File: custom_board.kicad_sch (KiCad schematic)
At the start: 20 parts, among them IC1 TMPM46BF10FG

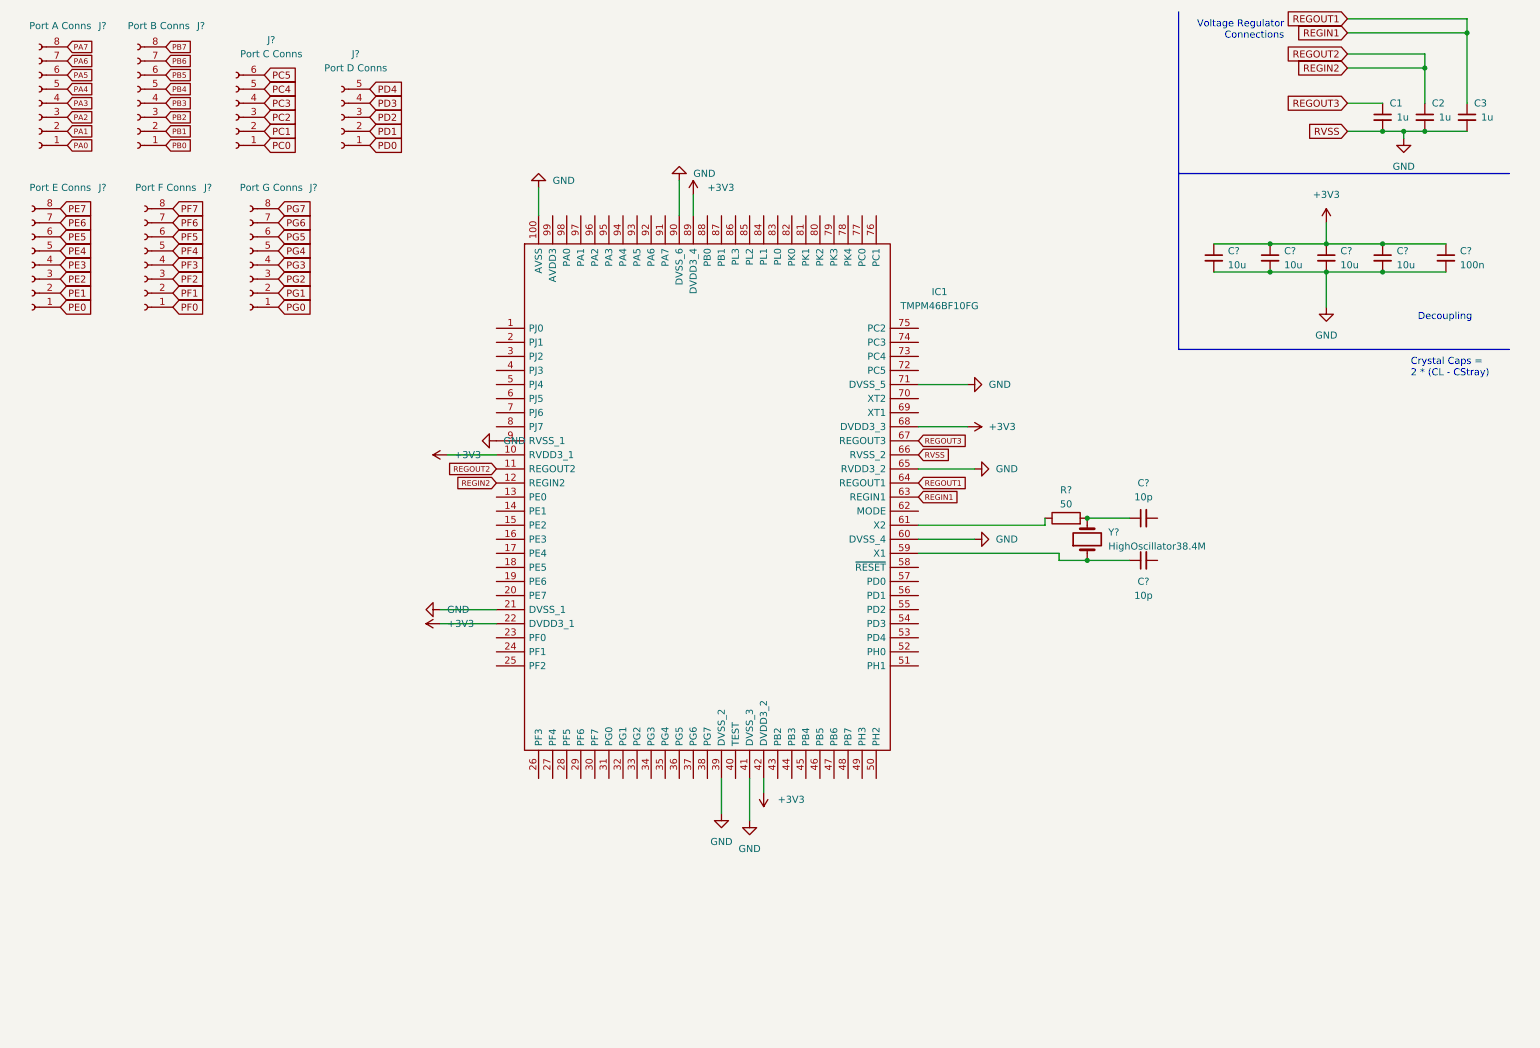
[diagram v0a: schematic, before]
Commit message: Update custom_board.kicad_sch
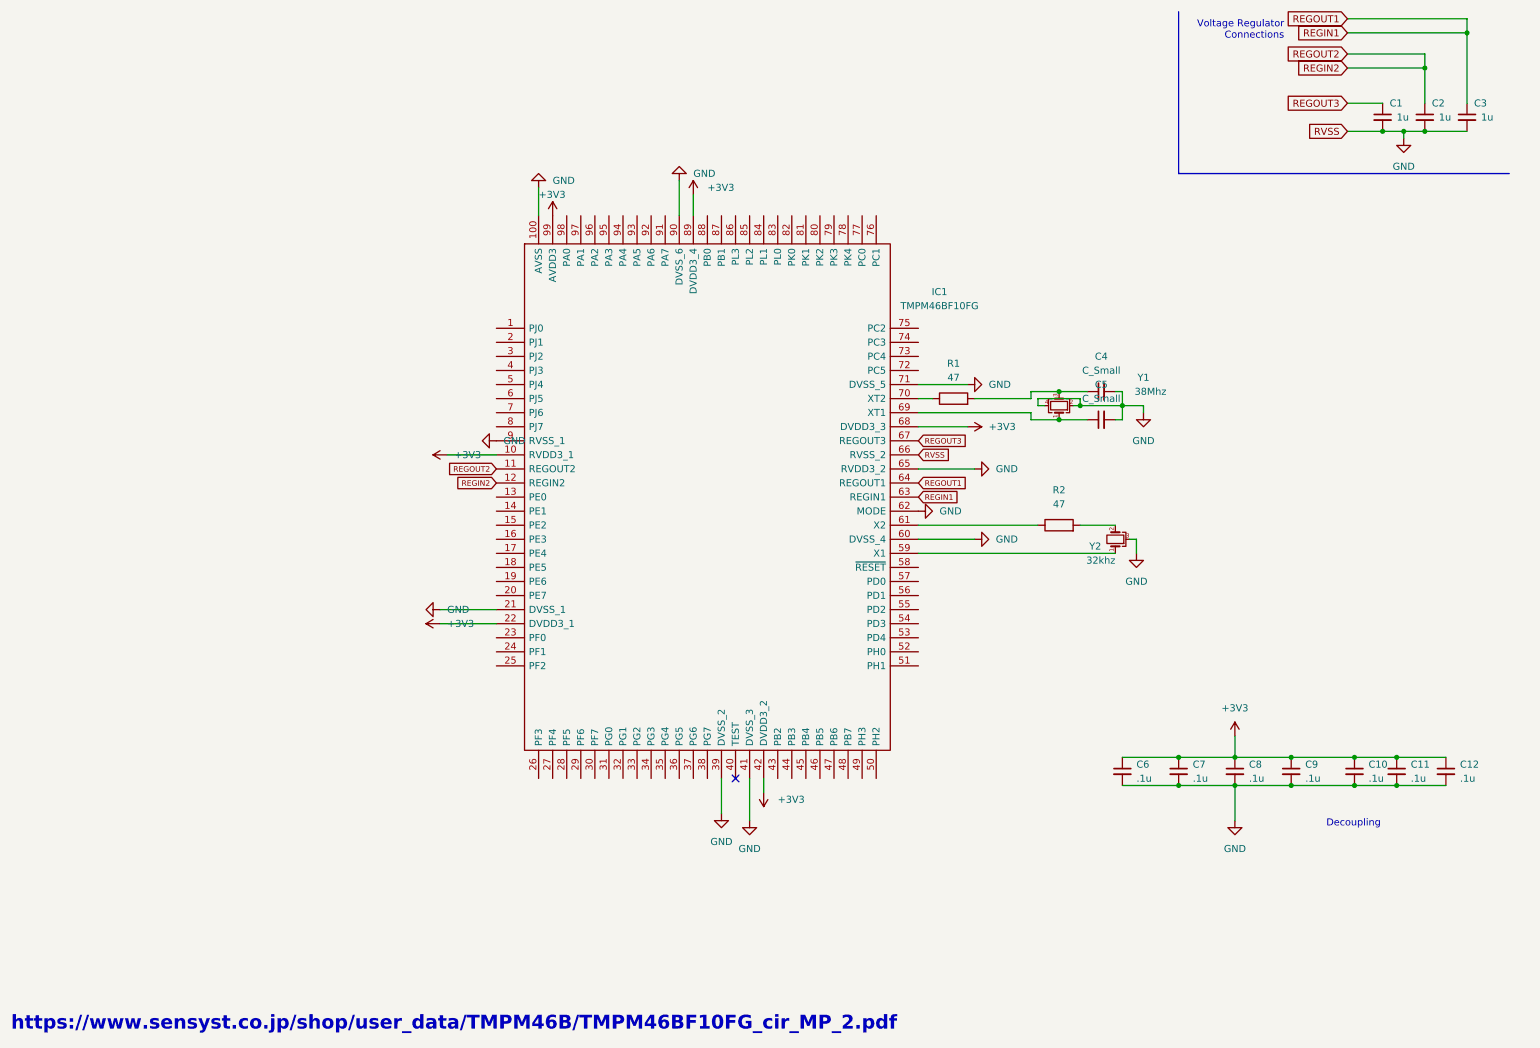
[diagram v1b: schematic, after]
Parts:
- removed C? (x2): 10p, symbol Device:C_Small
- removed C?: 100n, symbol Device:C_Small
- removed J?: Port A Conns, symbol Connector:Conn_01x08_Female
- removed J?: Port C Conns, symbol Connector:Conn_01x06_Female
- removed J?: Port F Conns, symbol Connector:Conn_01x08_Female
- removed J?: Port G Conns, symbol Connector:Conn_01x08_Female
- removed J?: Port B Conns, symbol Connector:Conn_01x08_Female
- removed J?: Port D Conns, symbol Connector:Conn_01x05_Female
- removed J?: Port E Conns, symbol Connector:Conn_01x08_Female
- removed R?: 50, symbol Device:R
- removed Y?: HighOscillator38.4M, symbol Device:Crystal
- added C10, C11, C12: .1u, symbol Device:C_Small
- added C4, C5: C_Small, symbol Device:C_Small
- added R1, R2: 47, symbol Device:R
- added Y1: 38Mhz, symbol Device:Crystal_GND24_Small
- added Y2: 32khz, symbol Device:Crystal_GND3_Small
- C6, C7, C8, C9: renamed from C?; value 10u -> .1u
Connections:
- net +3V3: now also IC1.99 (AVDD3), C10.1, C11.1, C12.1
- net GND: now also IC1.62 (MODE), C10.2, C11.2, C12.2, C4.2, C5.2, Y1.2, Y1.4, Y2.3
- net at IC1.59 (X1): now also Y2.1
- net at IC1.61 (X2): now also R2.1
- net at IC1.69 (XT1): now also C5.1, Y1.1
- net at IC1.70 (XT2): now also R1.1
- new net: R2.2, Y2.2
- new net: C4.1, R1.2, Y1.3
- no-connect marks 0 -> 1
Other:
- note added: "https://www.sensyst.co.jp/shop/user_data/TMPM46B/TMPM46BF10FG_cir_MP_2.pdf"
- note removed: "Crystal Caps = 2 * (CL - CStray)"
- moved on the sheet: C6, C7, C8, C9

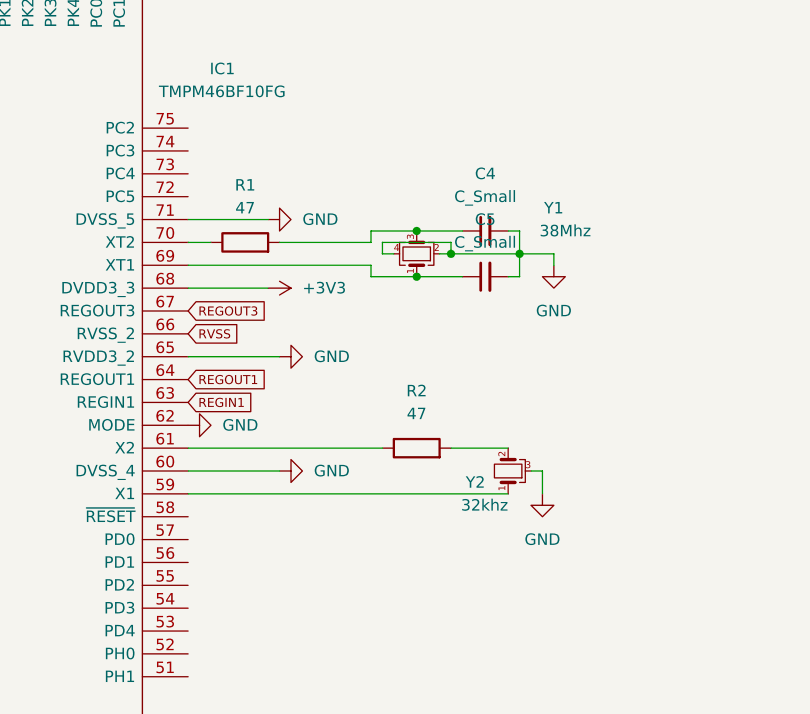
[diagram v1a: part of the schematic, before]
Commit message: Update custom_board.kicad_sch
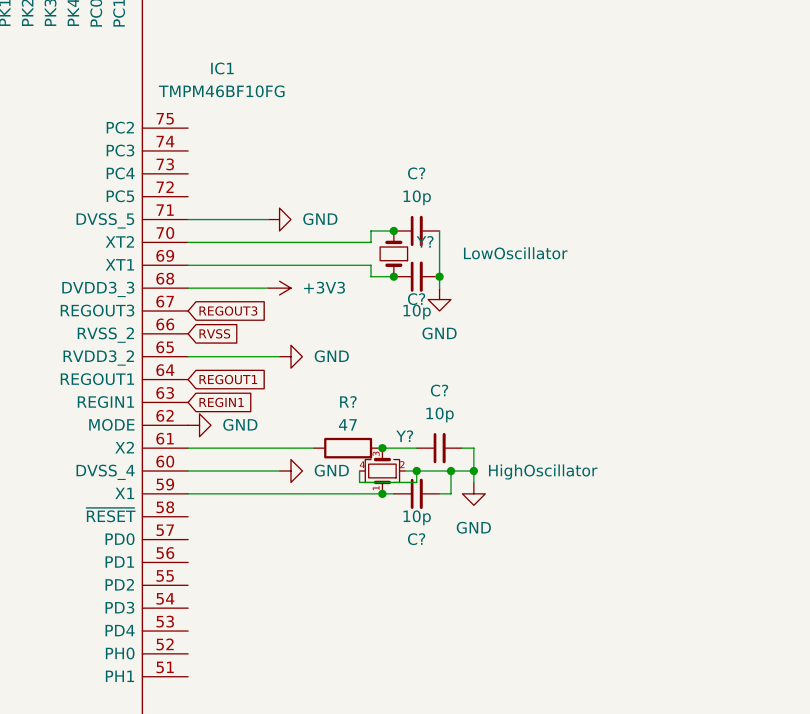
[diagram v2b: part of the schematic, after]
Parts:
- removed C4, C5: C_Small, symbol Device:C_Small
- removed R1, R2: 47, symbol Device:R
- removed Y1: 38Mhz, symbol Device:Crystal_GND24_Small
- removed Y2: 32khz, symbol Device:Crystal_GND3_Small
- added C? (x4): 10p, symbol Device:C_Small
- added R?: 47, symbol Device:R
- added Y?: LowOscillator, symbol Device:Crystal_Small
- added Y?: HighOscillator, symbol Device:Crystal_GND24_Small
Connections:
- net GND: now also C?.2, C?.2, C?.2, C?.2, Y?.2, Y?.4
- net at IC1.59 (X1): now also C?.1, Y?.1
- net at IC1.61 (X2): now also R?.1
- net at IC1.69 (XT1): now also C?.1, Y?.1
- net at IC1.70 (XT2): now also C?.1, Y?.2
- new net: C?.1, R?.2, Y?.3
